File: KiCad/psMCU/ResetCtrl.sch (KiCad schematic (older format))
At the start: 14 parts

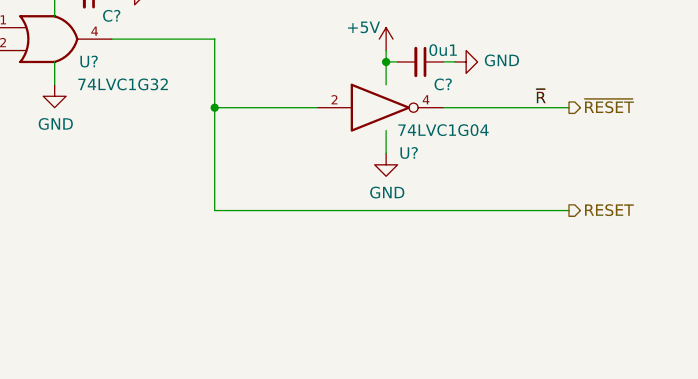
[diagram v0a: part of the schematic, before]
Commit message: Pulled in from clock test, root layout first draft
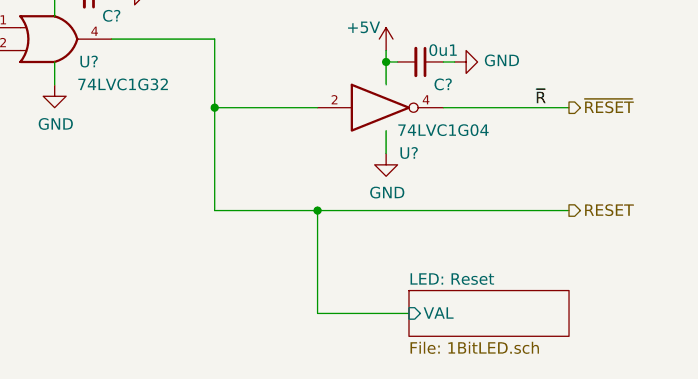
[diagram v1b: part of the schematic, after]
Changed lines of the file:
@@
 $Descr A4 11693 8268
 encoding utf-8
-Sheet 111 193
+Sheet 113 209
 Title "psMCU"
 Date ""
@@
 AR Path="/5F1CE57C/5FD43FAC" Ref="#PWR?"  Part="1"
 AR Path="/608BF85D/5FD43FAC" Ref="#PWR?"  Part="1"
-AR Path="/5FD3CD07/5FD43FAC" Ref="#PWR?"  Part="1"
-F 0 "#PWR?" H 8850 3100 50  0001 C CNN
+AR Path="/5FD3CD07/5FD43FAC" Ref="#PWR01660"  Part="1"
+F 0 "#PWR01660" H 8850 3100 50  0001 C CNN
 F 1 "GND" V 8855 3222 50  0000 R CNN
 F 2 "" H 8850 3350 50  0001 C CNN
@@
 AR Path="/5F1CE57C/5FD43FB4" Ref="#PWR?"  Part="1"
 AR Path="/608BF85D/5FD43FB4" Ref="#PWR?"  Part="1"
-AR Path="/5FD3CD07/5FD43FB4" Ref="#PWR?"  Part="1"
-F 0 "#PWR?" H 8550 3500 50  0001 C CNN
+AR Path="/5FD3CD07/5FD43FB4" Ref="#PWR01661"  Part="1"
+F 0 "#PWR01661" H 8550 3500 50  0001 C CNN
 F 1 "GND" H 8555 3577 50  0000 C CNN
 F 2 "" H 8550 3750 50  0001 C CNN
@@
 AR Path="/5F1CE57C/5FD43FC2" Ref="#PWR?"  Part="1"
 AR Path="/608BF85D/5FD43FC2" Ref="#PWR?"  Part="1"
-AR Path="/5FD3CD07/5FD43FC2" Ref="#PWR?"  Part="1"
-F 0 "#PWR?" H 8550 3150 50  0001 C CNN
+AR Path="/5FD3CD07/5FD43FC2" Ref="#PWR01662"  Part="1"
+F 0 "#PWR01662" H 8550 3150 50  0001 C CNN
 F 1 "+5V" H 8450 3400 50  0000 C CNN
 F 2 "" H 8550 3300 50  0001 C CNN
@@
 	8800 3550 9350 3550
 Wire Wire Line
-	9350 4000 7800 4000
+	9350 4000 8250 4000
 Wire Wire Line
 	7800 4000 7800 3550
@@
 AR Path="/5F1CE57C/5FF7364D" Ref="#PWR?"  Part="1"
 AR Path="/5F396002/5FF7364D" Ref="#PWR?"  Part="1"
-AR Path="/5FD3CD07/5FF7364D" Ref="#PWR?"  Part="1"
-F 0 "#PWR?" H 5850 3150 50  0001 C CNN
+AR Path="/5FD3CD07/5FF7364D" Ref="#PWR01663"  Part="1"
+F 0 "#PWR01663" H 5850 3150 50  0001 C CNN
 F 1 "GND" H 5855 3227 50  0000 C CNN
 F 2 "" H 5850 3400 50  0001 C CNN
@@
 AR Path="/5F1CE57C/5FF73655" Ref="#PWR?"  Part="1"
 AR Path="/5F396002/5FF73655" Ref="#PWR?"  Part="1"
-AR Path="/5FD3CD07/5FF73655" Ref="#PWR?"  Part="1"
-F 0 "#PWR?" H 5850 2800 50  0001 C CNN
+AR Path="/5FD3CD07/5FF73655" Ref="#PWR01664"  Part="1"
+F 0 "#PWR01664" H 5850 2800 50  0001 C CNN
 F 1 "+5V" H 5865 3123 50  0000 C CNN
 F 2 "" H 5850 2950 50  0001 C CNN
@@
 AR Path="/5F1CE57C/5FF73664" Ref="#PWR?"  Part="1"
 AR Path="/5F396002/5FF73664" Ref="#PWR?"  Part="1"
-AR Path="/5FD3CD07/5FF73664" Ref="#PWR?"  Part="1"
-F 0 "#PWR?" H 6150 2750 50  0001 C CNN
+AR Path="/5FD3CD07/5FF73664" Ref="#PWR01665"  Part="1"
+F 0 "#PWR01665" H 6150 2750 50  0001 C CNN
 F 1 "GND" V 6155 2872 50  0000 R CNN
 F 2 "" H 6150 3000 50  0001 C CNN
@@
 AR Path="/5F1CE57C/5FFDD1F3" Ref="#PWR?"  Part="1"
 AR Path="/5F396002/5FFDD1F3" Ref="#PWR?"  Part="1"
-AR Path="/5FD3CD07/5FFDD1F3" Ref="#PWR?"  Part="1"
-F 0 "#PWR?" H 3450 2700 50  0001 C CNN
+AR Path="/5FD3CD07/5FFDD1F3" Ref="#PWR01666"  Part="1"
+F 0 "#PWR01666" H 3450 2700 50  0001 C CNN
 F 1 "GND" V 3455 2822 50  0000 R CNN
 F 2 "" H 3450 2950 50  0001 C CNN
@@
 AR Path="/5F1CE57C/5FFDD202" Ref="#PWR?"  Part="1"
 AR Path="/5F396002/5FFDD202" Ref="#PWR?"  Part="1"
-AR Path="/5FD3CD07/5FFDD202" Ref="#PWR?"  Part="1"
-F 0 "#PWR?" H 3150 2750 50  0001 C CNN
+AR Path="/5FD3CD07/5FFDD202" Ref="#PWR01667"  Part="1"
+F 0 "#PWR01667" H 3150 2750 50  0001 C CNN
 F 1 "+5V" H 3165 3073 50  0000 C CNN
 F 2 "" H 3150 2900 50  0001 C CNN
@@
 AR Path="/5F1CE57C/5FFDD209" Ref="#PWR?"  Part="1"
 AR Path="/5F396002/5FFDD209" Ref="#PWR?"  Part="1"
-AR Path="/5FD3CD07/5FFDD209" Ref="#PWR?"  Part="1"
-F 0 "#PWR?" H 3150 3050 50  0001 C CNN
+AR Path="/5FD3CD07/5FFDD209" Ref="#PWR01668"  Part="1"
+F 0 "#PWR01668" H 3150 3050 50  0001 C CNN
 F 1 "GND" H 3250 3150 50  0000 R CNN
 F 2 "" H 3150 3300 50  0001 C CNN
@@
 AR Path="/5F1CE57C/5FFDEBBC" Ref="#PWR?"  Part="1"
 AR Path="/5F396002/5FFDEBBC" Ref="#PWR?"  Part="1"
-AR Path="/5FD3CD07/5FFDEBBC" Ref="#PWR?"  Part="1"
-F 0 "#PWR?" H 2400 3250 50  0001 C CNN
+AR Path="/5FD3CD07/5FFDEBBC" Ref="#PWR01669"  Part="1"
+F 0 "#PWR01669" H 2400 3250 50  0001 C CNN
 F 1 "GND" H 2500 3350 50  0000 R CNN
 F 2 "" H 2400 3500 50  0001 C CNN
@@
 AR Path="/5F1CE57C/5FFE9777" Ref="#PWR?"  Part="1"
 AR Path="/5F396002/5FFE9777" Ref="#PWR?"  Part="1"
-AR Path="/5FD3CD07/5FFE9777" Ref="#PWR?"  Part="1"
-F 0 "#PWR?" H 2400 2350 50  0001 C CNN
+AR Path="/5FD3CD07/5FFE9777" Ref="#PWR01670"  Part="1"
+F 0 "#PWR01670" H 2400 2350 50  0001 C CNN
 F 1 "+5V" H 2415 2673 50  0000 C CNN
 F 2 "" H 2400 2500 50  0001 C CNN
@@
 AR Path="/5F1CE57C/6000A97B" Ref="#PWR?"  Part="1"
 AR Path="/608BF85D/6000A97B" Ref="#PWR?"  Part="1"
-AR Path="/5FD3CD07/6000A97B" Ref="#PWR?"  Part="1"
-F 0 "#PWR?" H 4300 2700 50  0001 C CNN
+AR Path="/5FD3CD07/6000A97B" Ref="#PWR01671"  Part="1"
+F 0 "#PWR01671" H 4300 2700 50  0001 C CNN
 F 1 "GND" V 4305 2822 50  0000 R CNN
 F 2 "" H 4300 2950 50  0001 C CNN
@@
 AR Path="/5F1CE57C/6000A983" Ref="#PWR?"  Part="1"
 AR Path="/608BF85D/6000A983" Ref="#PWR?"  Part="1"
-AR Path="/5FD3CD07/6000A983" Ref="#PWR?"  Part="1"
-F 0 "#PWR?" H 4000 3100 50  0001 C CNN
+AR Path="/5FD3CD07/6000A983" Ref="#PWR01672"  Part="1"
+F 0 "#PWR01672" H 4000 3100 50  0001 C CNN
 F 1 "GND" H 4005 3177 50  0000 C CNN
 F 2 "" H 4000 3350 50  0001 C CNN
@@
 AR Path="/5F1CE57C/6000A991" Ref="#PWR?"  Part="1"
 AR Path="/608BF85D/6000A991" Ref="#PWR?"  Part="1"
-AR Path="/5FD3CD07/6000A991" Ref="#PWR?"  Part="1"
-F 0 "#PWR?" H 4000 2750 50  0001 C CNN
+AR Path="/5FD3CD07/6000A991" Ref="#PWR01673"  Part="1"
+F 0 "#PWR01673" H 4000 2750 50  0001 C CNN
 F 1 "+5V" H 3900 3000 50  0000 C CNN
 F 2 "" H 4000 2900 50  0001 C CNN
@@
 AR Path="/5F1CE57C/61C134A2" Ref="#PWR?"  Part="1"
 AR Path="/5F396002/61C134A2" Ref="#PWR?"  Part="1"
-AR Path="/5FD3CD07/61C134A2" Ref="#PWR?"  Part="1"
-F 0 "#PWR?" H 7100 3200 50  0001 C CNN
+AR Path="/5FD3CD07/61C134A2" Ref="#PWR01674"  Part="1"
+F 0 "#PWR01674" H 7100 3200 50  0001 C CNN
 F 1 "GND" H 7105 3277 50  0000 C CNN
 F 2 "" H 7100 3450 50  0001 C CNN
@@
 AR Path="/5F1CE57C/61C134AA" Ref="#PWR?"  Part="1"
 AR Path="/5F396002/61C134AA" Ref="#PWR?"  Part="1"
-AR Path="/5FD3CD07/61C134AA" Ref="#PWR?"  Part="1"
-F 0 "#PWR?" H 7100 2850 50  0001 C CNN
+AR Path="/5FD3CD07/61C134AA" Ref="#PWR01675"  Part="1"
+F 0 "#PWR01675" H 7100 2850 50  0001 C CNN
 F 1 "+5V" H 7115 3173 50  0000 C CNN
 F 2 "" H 7100 3000 50  0001 C CNN
@@
 AR Path="/5F1CE57C/61C134B9" Ref="#PWR?"  Part="1"
 AR Path="/5F396002/61C134B9" Ref="#PWR?"  Part="1"
-AR Path="/5FD3CD07/61C134B9" Ref="#PWR?"  Part="1"
-F 0 "#PWR?" H 7400 2800 50  0001 C CNN
+AR Path="/5FD3CD07/61C134B9" Ref="#PWR01676"  Part="1"
+F 0 "#PWR01676" H 7400 2800 50  0001 C CNN
 F 1 "GND" V 7405 2922 50  0000 R CNN
 F 2 "" H 7400 3050 50  0001 C CNN
@@
 Wire Wire Line
 	5300 3150 5550 3150
+$Sheet
+S 8650 4350 700  200
+U 602A39E5
+F0 "LED: Reset" 50
+F1 "1BitLED.sch" 50
+F2 "VAL" I L 8650 4450 50
+$EndSheet
+Wire Wire Line
+	8650 4450 8250 4450
+Wire Wire Line
+	8250 4450 8250 4000
+Connection ~ 8250 4000
+Wire Wire Line
+	8250 4000 7800 4000
 $EndSCHEMATC
